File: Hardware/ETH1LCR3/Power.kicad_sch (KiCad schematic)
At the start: 57 parts, among them Q401 SI5618A, Q402 MMBT3904, Q403 BSS123, U401 REG103GA-3.3, U402 LT1946A, U403 REG103GA-5, U404 TEL5-2411, U405 LT1611

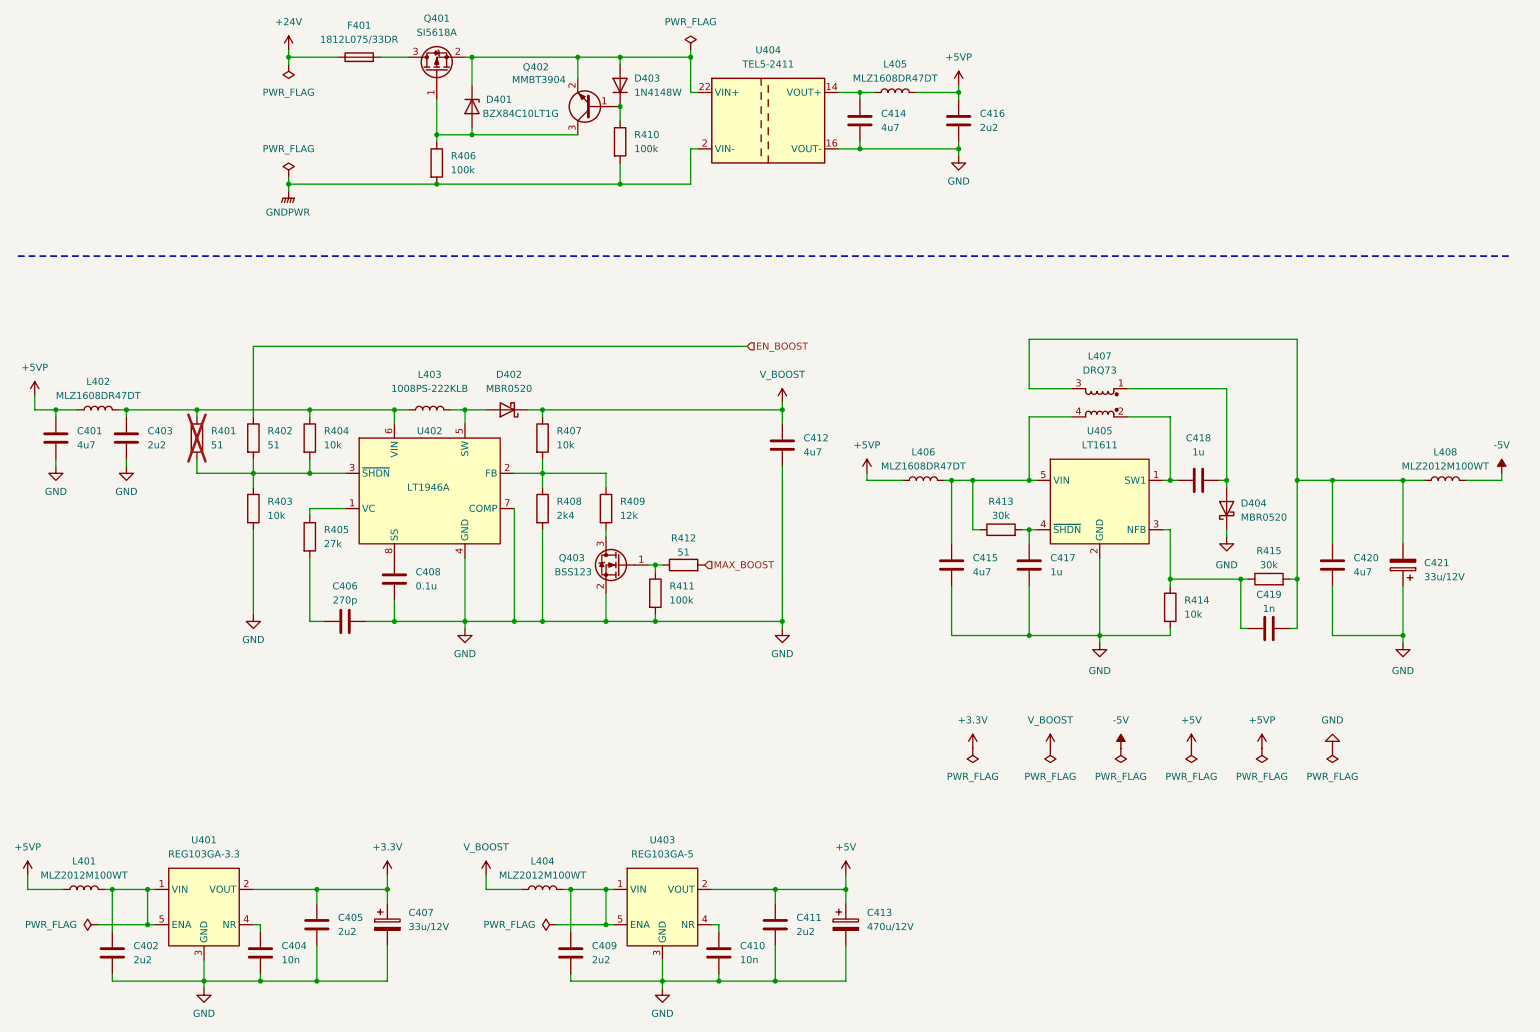
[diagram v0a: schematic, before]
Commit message: Hardware
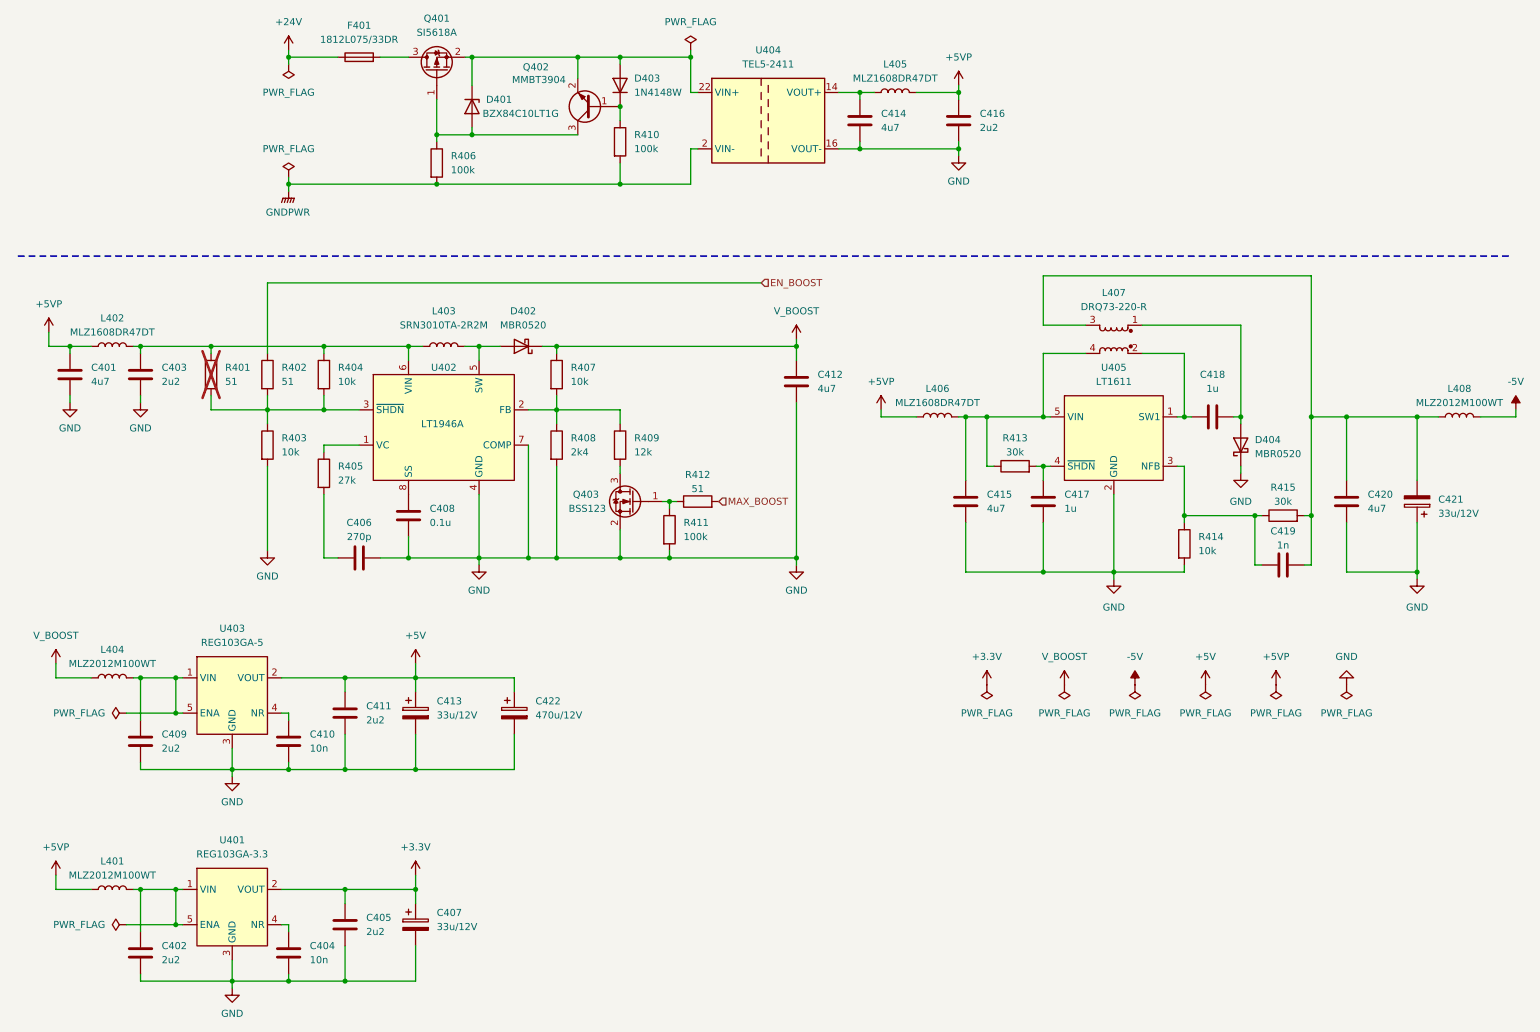
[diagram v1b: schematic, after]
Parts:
- added C422: 470u/12V, Capacitor_SMD:CP_Elec_10x10.5, symbol Device:C_Polarized
- C401, C402, C403, C405, C409, C411, C412, C414, C415, C416, C420: footprint (none) -> Capacitor_SMD:C_0805_2012Metric_Pad1.18x1.45mm_HandSolder
- C407, C421: footprint (none) -> Capacitor_Tantalum_SMD:CP_EIA-3528-21_Kemet-B_Pad1.50x2.35mm_HandSolder
- C413: value 470u/12V -> 33u/12V; footprint (none) -> Capacitor_Tantalum_SMD:CP_EIA-3528-21_Kemet-B_Pad1.50x2.35mm_HandSolder
- D402, D404: footprint (none) -> Diode_SMD:D_SOD-123F
- L403: value 1008PS-222KLB -> SRN3010TA-2R2M
- L407: value DRQ73 -> DRQ73-220-R; footprint (none) -> ETH1LCR3:DRQ73
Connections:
- net +5V: now also C422.1
- net GND: now also C422.2
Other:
- moved on the sheet: C401, C402, C403, C404, C405, C406, C407, C408, C409, C410, C411, C412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
